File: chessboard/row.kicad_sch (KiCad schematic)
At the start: 15 parts, among them U1 TCA9548APWR

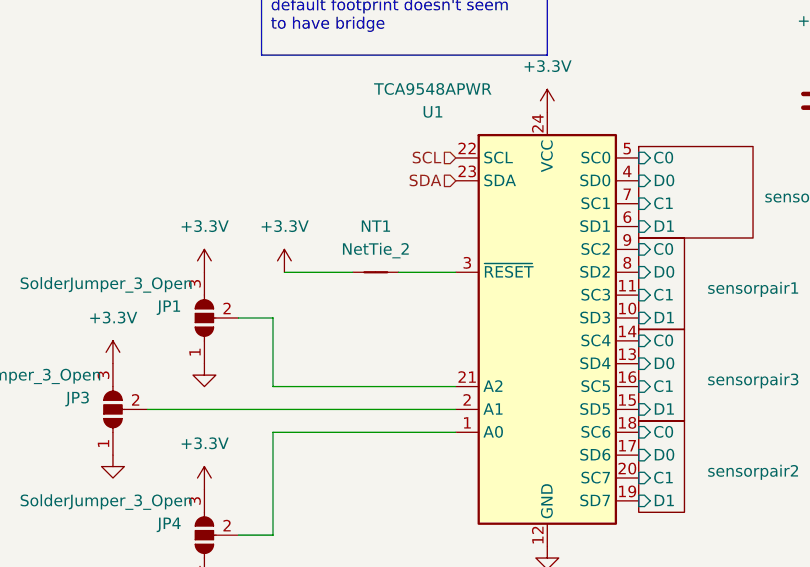
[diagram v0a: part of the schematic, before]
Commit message: ready to buy
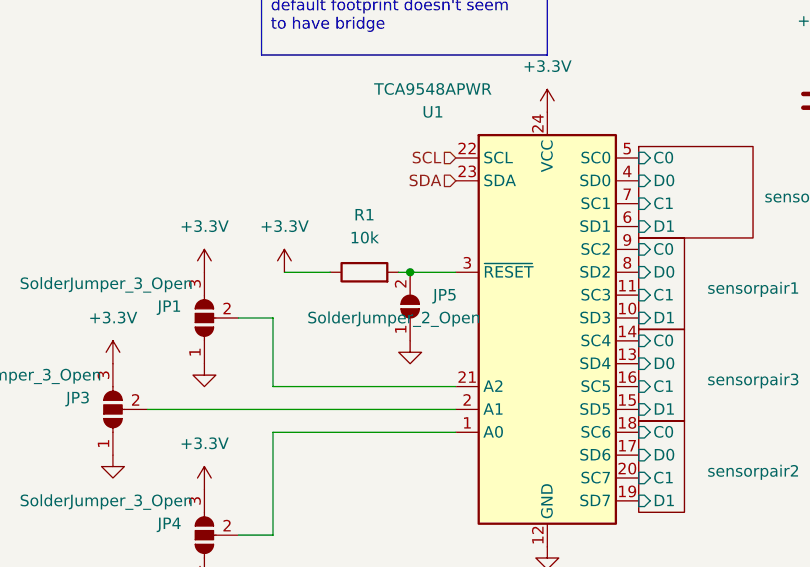
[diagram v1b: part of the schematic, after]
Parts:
- removed NT1: NetTie_2, Jumper:SolderJumper-2_P1.3mm_Bridged_Pad1.0x1.5mm, symbol Device:NetTie_2
- added JP5: SolderJumper_2_Open, Jumper:SolderJumper-2_P1.3mm_Open_Pad1.0x1.5mm, symbol Jumper:SolderJumper_2_Open
- added R1: 10k, Resistor_SMD:R_0805_2012Metric_Pad1.20x1.40mm_HandSolder, symbol Device:R
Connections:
- net +3.3V: now also R1.1
- net GND: now also JP5.1 (A)
- net at U1.3 (~{RESET}): now also JP5.2 (B), R1.2
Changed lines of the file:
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@@
   (junction (at 160.02 74.93) (diameter 0) (color 0 0 0 0)
   )
+  (junction (at 74.93 139.7) (diameter 0) (color 0 0 0 0)
+  )
   (junction (at 220.98 59.69) (diameter 0) (color 0 0 0 0)
   )
@@
     (stroke (width 0) (type default))
   )
-  (wire (pts (xy 73.66 139.7) (xy 80.01 139.7))
+  (wire (pts (xy 73.66 139.7) (xy 74.93 139.7))
     (stroke (width 0) (type default))
   )
@@
     (stroke (width 0) (type default))
   )
+  (wire (pts (xy 74.93 139.7) (xy 80.01 139.7))
+    (stroke (width 0) (type default))
+  )
   (wire (pts (xy 190.5 59.69) (xy 205.74 59.69))
     (stroke (width 0) (type default))
@@
     (stroke (width 0) (type default))
   )
-  (wire (pts (xy 60.96 139.7) (xy 68.58 139.7))
+  (wire (pts (xy 60.96 139.7) (xy 66.04 139.7))
     (stroke (width 0) (type default))
   )
@@
     )
   )
-  (symbol (lib_id "Device:NetTie_2") (at 71.12 139.7 0) (unit 1)
-    (in_bom no) (on_board yes) (dnp no) (fields_autoplaced)
-    (property "Reference" "NT1" (at 71.12 134.62 0)
-      (effects (font (size 1.27 1.27)))
-    )
-    (property "Value" "NetTie_2" (at 71.12 137.16 0)
-      (effects (font (size 1.27 1.27)))
-    )
-    (property "Footprint" "Jumper:SolderJumper-2_P1.3mm_Bridged_Pad1.0x1.5mm" (at 71.12 139.7 0)
-      (effects (font (size 1.27 1.27)) hide)
-    )
-    (property "Datasheet" "~" (at 71.12 139.7 0)
-      (effects (font (size 1.27 1.27)) hide)
-    )
-    (pin "1")
-    (pin "2")
-    (instances
-      (project "chessboard"
-        (path "/178674ef-da23-4447-9d4b-ea3429461404/501c11bc-04bd-4d54-8bc8-c6f63ce2a0b8"
-          (reference "NT1") (unit 1)
+  (symbol (lib_id "Device:R") (at 69.85 139.7 90) (unit 1)
+    (in_bom yes) (on_board yes) (dnp no) (fields_autoplaced)
+    (property "Reference" "R1" (at 69.85 133.35 90)
+      (effects (font (size 1.27 1.27)))
+    )
+    (property "Value" "10k" (at 69.85 135.89 90)
+      (effects (font (size 1.27 1.27)))
+    )
+    (property "Footprint" "Resistor_SMD:R_0805_2012Metric_Pad1.20x1.40mm_HandSolder" (at 69.85 141.478 90)
+      (effects (font (size 1.27 1.27)) hide)
+    )
+    (property "Datasheet" "~" (at 69.85 139.7 0)
+      (effects (font (size 1.27 1.27)) hide)
+    )
+    (pin "1")
+    (pin "2")
+    (instances
+      (project "chessboard"
+        (path "/178674ef-da23-4447-9d4b-ea3429461404/501c11bc-04bd-4d54-8bc8-c6f63ce2a0b8"
+          (reference "R1") (unit 1)
         )
       )
@@
     )
   )
+  (symbol (lib_id "power:GND") (at 74.93 147.32 0) (unit 1)
+    (in_bom yes) (on_board yes) (dnp no) (fields_autoplaced)
+    (property "Reference" "#PWR010" (at 74.93 153.67 0)
+      (effects (font (size 1.27 1.27)) hide)
+    )
+    (property "Value" "GND" (at 74.93 152.4 0)
+      (effects (font (size 1.27 1.27)) hide)
+    )
+    (property "Footprint" "" (at 74.93 147.32 0)
+      (effects (font (size 1.27 1.27)) hide)
+    )
+    (property "Datasheet" "" (at 74.93 147.32 0)
+      (effects (font (size 1.27 1.27)) hide)
+    )
+    (pin "1")
+    (instances
+      (project "chessboard"
+        (path "/178674ef-da23-4447-9d4b-ea3429461404"
+          (reference "#PWR010") (unit 1)
+        )
+        (path "/178674ef-da23-4447-9d4b-ea3429461404/501c11bc-04bd-4d54-8bc8-c6f63ce2a0b8"
+          (reference "#PWR042") (unit 1)
+        )
+      )
+    )
+  )
   (symbol (lib_id "power:GND") (at 41.91 160.02 0) (unit 1)
     (in_bom yes) (on_board yes) (dnp no) (fields_autoplaced)
@@
         )
       )
+    )
+  )
+  (symbol (lib_id "Jumper:SolderJumper_2_Open") (at 74.93 143.51 270) (mirror x) (unit 1)
+    (in_bom yes) (on_board yes) (dnp no)
+    (property "Reference" "JP5" (at 77.47 142.24 90)
+      (effects (font (size 1.27 1.27)) (justify left))
+    )
+    (property "Value" "SolderJumper_2_Open" (at 63.5 144.78 90)
+      (effects (font (size 1.27 1.27)) (justify left))
+    )
+    (property "Footprint" "Jumper:SolderJumper-2_P1.3mm_Open_Pad1.0x1.5mm" (at 74.93 143.51 0)
+      (effects (font (size 1.27 1.27)) hide)
+    )
+    (property "Datasheet" "~" (at 74.93 143.51 0)
+      (effects (font (size 1.27 1.27)) hide)
+    )
+    (pin "2")
+    (pin "1")
+    (instances
+      (project "chessboard"
+        (path "/178674ef-da23-4447-9d4b-ea3429461404/501c11bc-04bd-4d54-8bc8-c6f63ce2a0b8"
+          (reference "JP5") (unit 1)
+        )
+      )
